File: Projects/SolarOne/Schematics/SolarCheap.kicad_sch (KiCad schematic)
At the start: 41 parts, among them J1 Solar, J2 Batt_Test, J3 USB_C_Receptacle, J4 1PPS, J5 Conn_01x02, J6 Conn_01x02, J7 Conn_01x04, J8 Conn_01x04, Q2 AO3401A, U1 CN3791, U2 HT-CT62, U3 TLV1117-33, U4 TMP102xxDRL, U5 ATGM336H

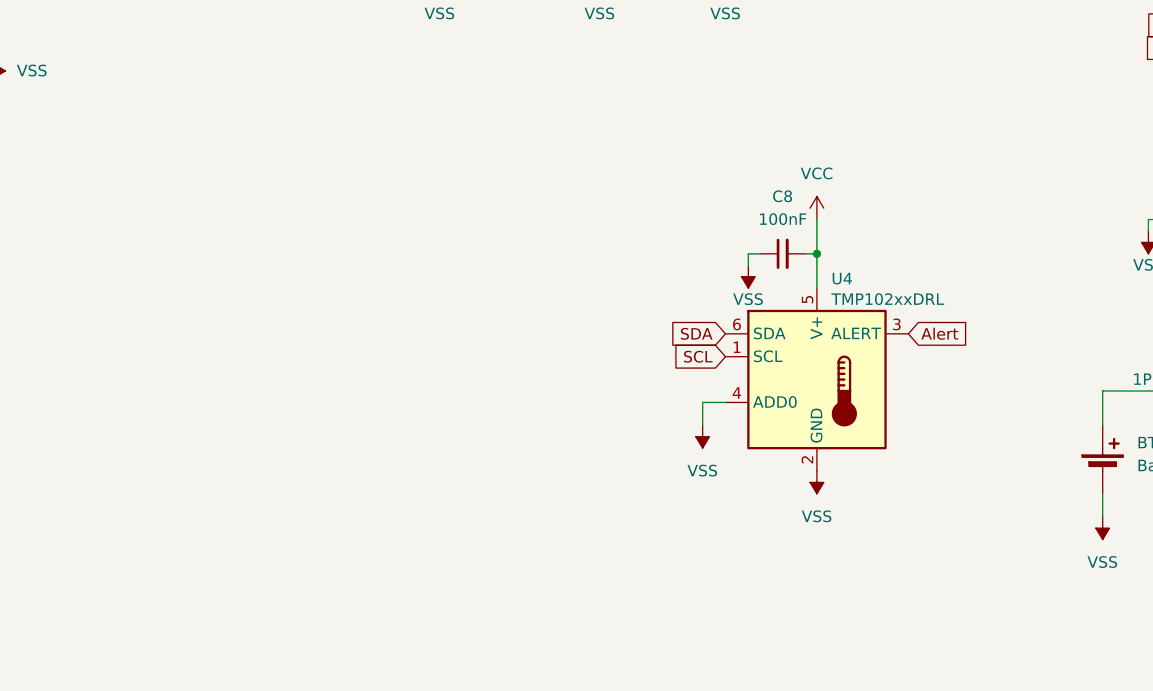
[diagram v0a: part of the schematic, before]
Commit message: Fixed SolarOne and other
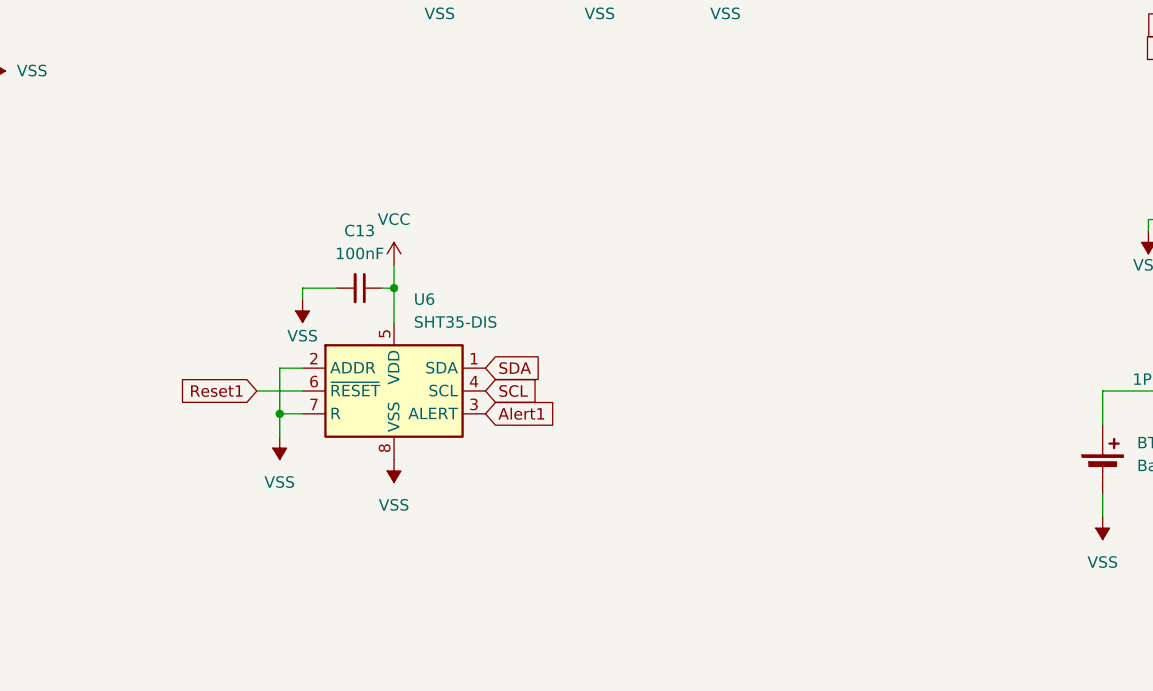
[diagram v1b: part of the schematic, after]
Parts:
- removed C8: 100nF, Capacitor_SMD:C_0805_2012Metric, symbol Device:C_Small
- removed U4: TMP102xxDRL, Package_TO_SOT_SMD:SOT-563, symbol Sensor_Temperature:TMP102xxDRL
- added C13: 100nF, Capacitor_SMD:C_0805_2012Metric, symbol Device:C_Small
- added U6: SHT35-DIS, Sensor_Humidity:Sensirion_DFN-8-1EP_2.5x2.5mm_P0.5mm_EP1.1x1.7mm, symbol Sensor_Humidity:SHT35-DIS
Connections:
- net SCL: now also U6.4 (SCL)
- net SDA: now also U6.1 (SDA)
- net VCC: now also C13.1, U6.5 (VDD)
- net VSS: now also C13.2, U6.2 (ADDR), U6.7 (R), U6.8 (VSS), U6.9 (VSS)
- new net Alert1: U6.3 (ALERT)
- new net Reset1: U6.6 (~{RESET})
